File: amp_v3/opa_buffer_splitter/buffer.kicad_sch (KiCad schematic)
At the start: 17 parts, among them J11 AUDIO_IN, J12 AUDIO_OUT, J15 OP_PWR_POS, J16 OP_PWR_NEG, U3 OPA1656

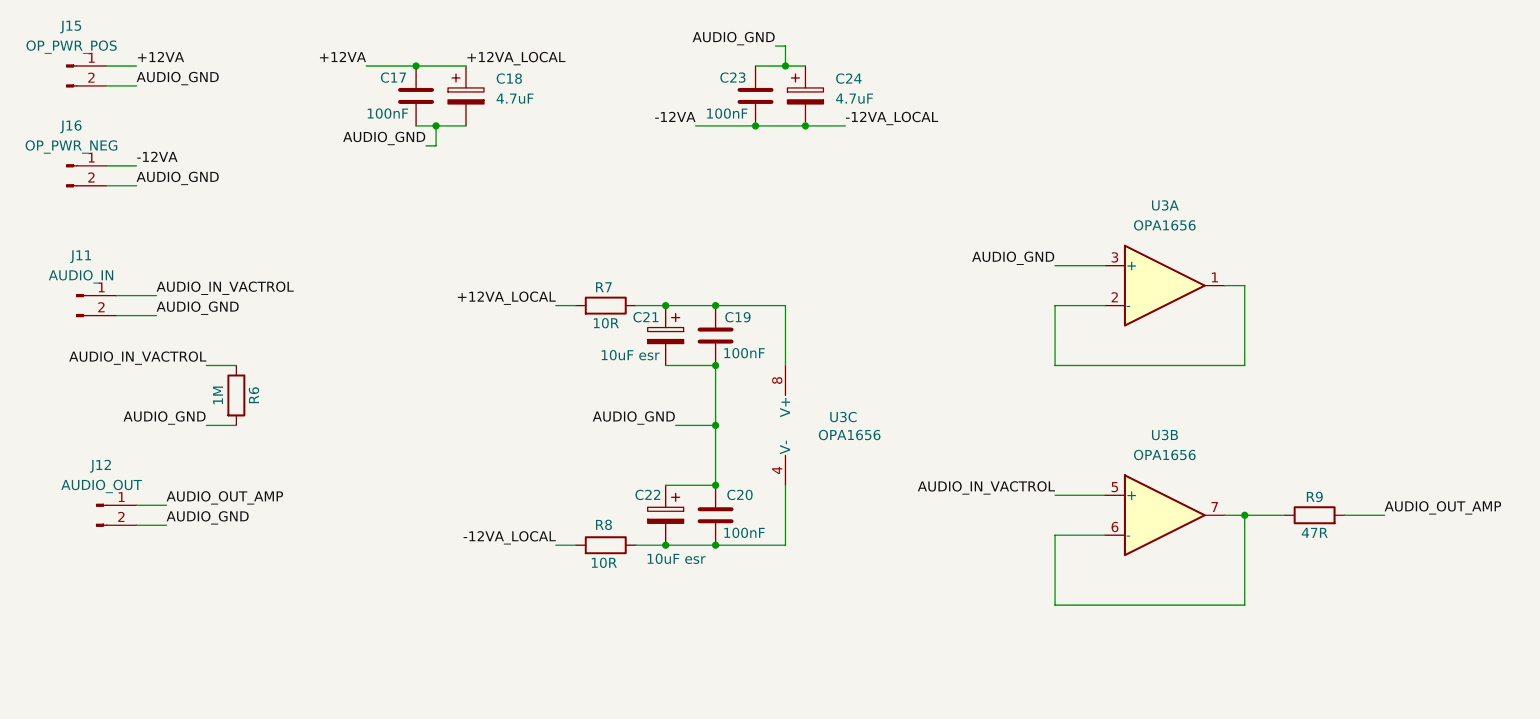
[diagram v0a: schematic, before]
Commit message: updates
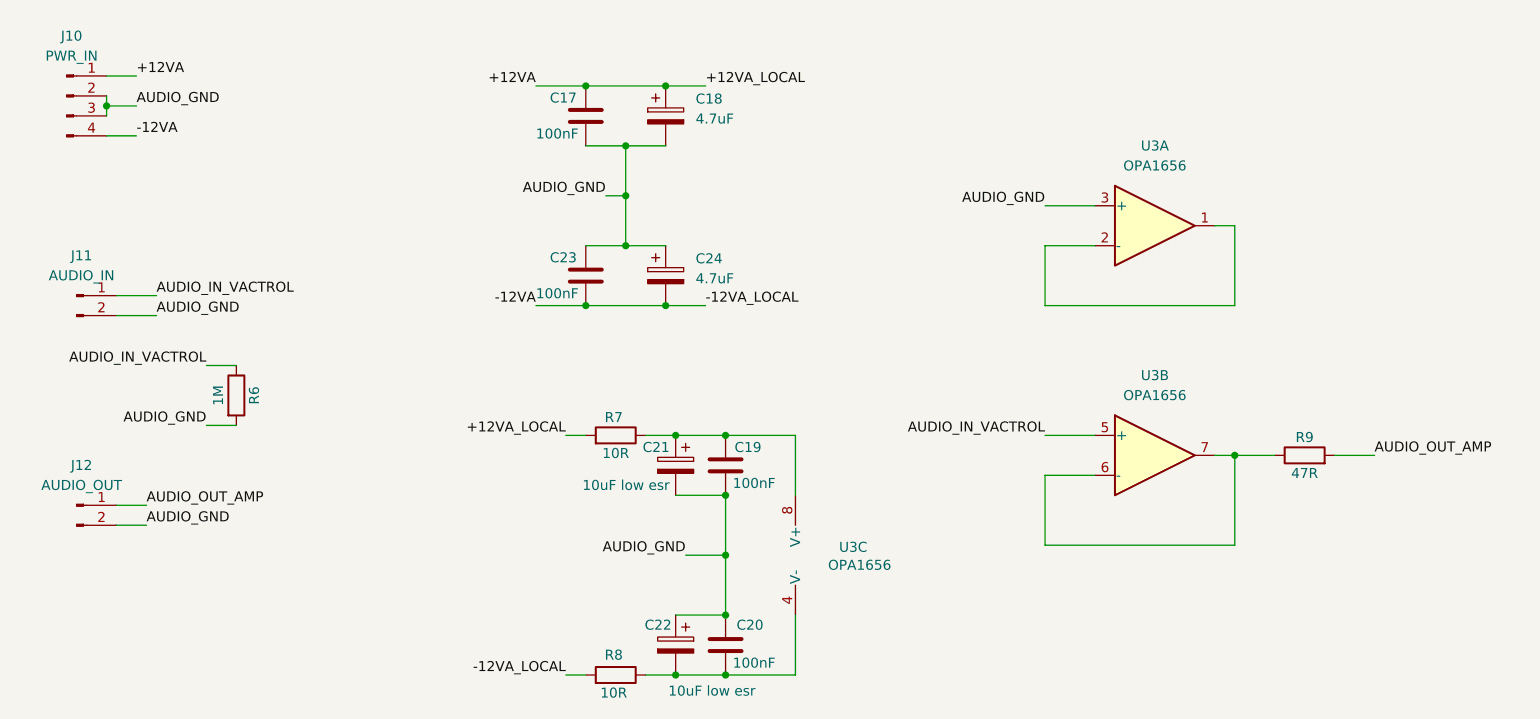
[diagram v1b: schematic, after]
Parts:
- removed J15: OP_PWR_POS, Connector_JST:JST_XH_B2B-XH-A_1x02_P2.50mm_Vertical, symbol Connector:Conn_01x02_Pin
- removed J16: OP_PWR_NEG, Connector_JST:JST_XH_B2B-XH-A_1x02_P2.50mm_Vertical, symbol Connector:Conn_01x02_Pin
- added J10: PWR_IN, Connector_JST:JST_XH_B4B-XH-A_1x04_P2.50mm_Vertical, symbol Connector:Conn_01x04_Pin
- C21, C22: value 10uF esr -> 10uF low esr
- R6: footprint Resistor_THT:R_Axial_DIN0207_L6.3mm_D2.5mm_P2.54mm_Vertical -> Resistor_THT:R_Axial_DIN0207_L6.3mm_D2.5mm_P7.62mm_Horizontal
- R7, R8: footprint Resistor_THT:R_Axial_DIN0207_L6.3mm_D2.5mm_P10.16mm_Horizontal -> Resistor_THT:R_Axial_DIN0207_L6.3mm_D2.5mm_P7.62mm_Horizontal
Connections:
- net +12VA: now also J10.1 (Pin_1)
- net -12VA: now also J10.4 (Pin_4)
- net AUDIO_GND: now also J10.2 (Pin_2), J10.3 (Pin_3)
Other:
- moved on the sheet: C17, C18, C19, C20, C21, C22, C23, C24, J12, R7, R8, R9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
